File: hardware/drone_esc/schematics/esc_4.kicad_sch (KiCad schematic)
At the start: 32 parts, among them Q19 BSC016N04LS, Q20 BSC016N04LS, Q21 BSC016N04LS, Q22 BSC016N04LS, Q23 BSC016N04LS, Q24 BSC016N04LS, U10 FD6288Q

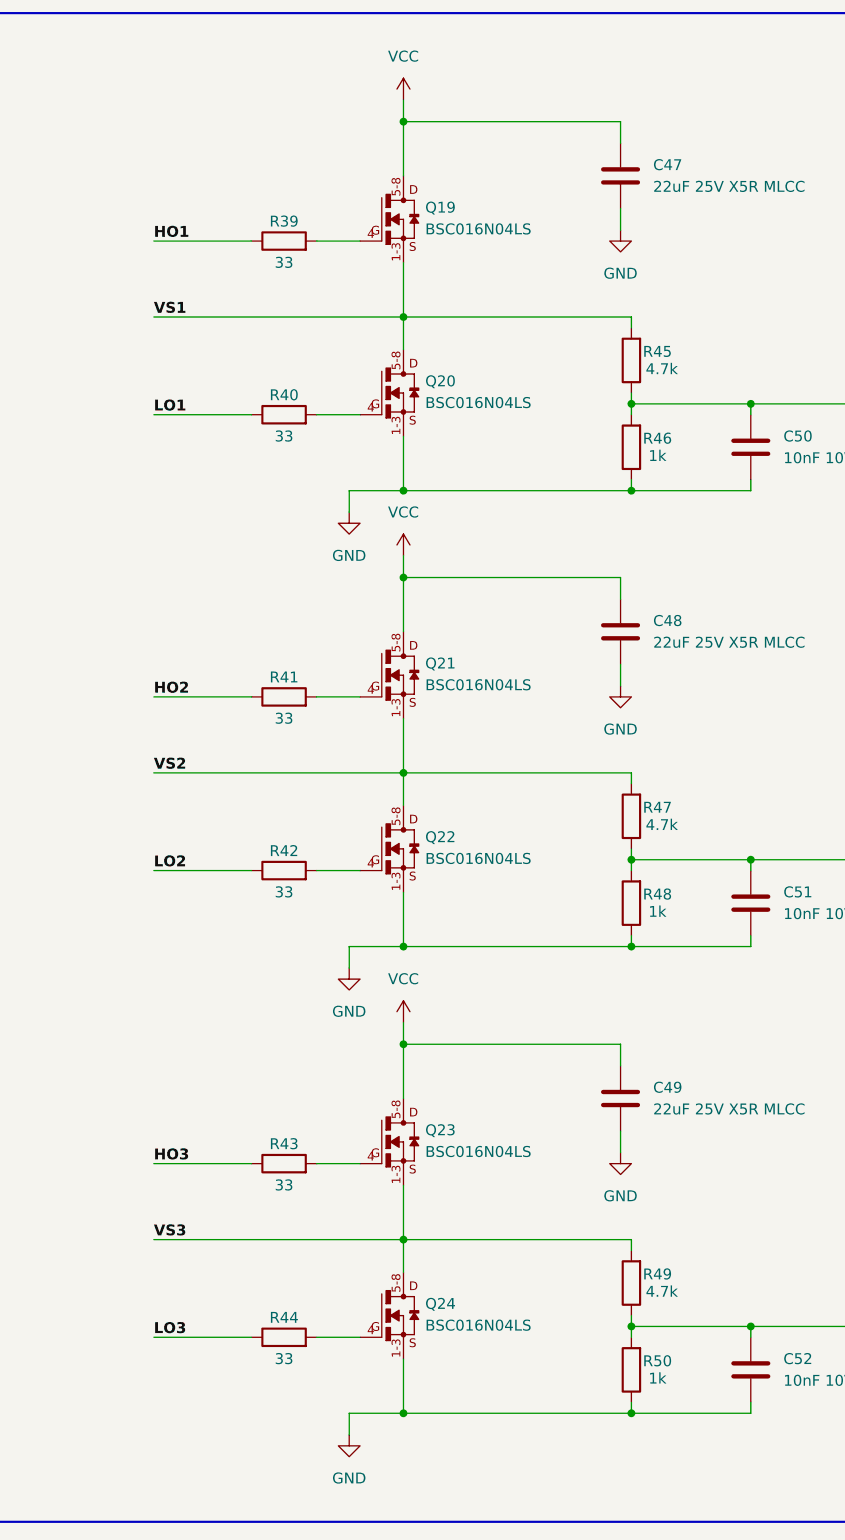
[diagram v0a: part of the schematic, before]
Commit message: replaced some of the schematics
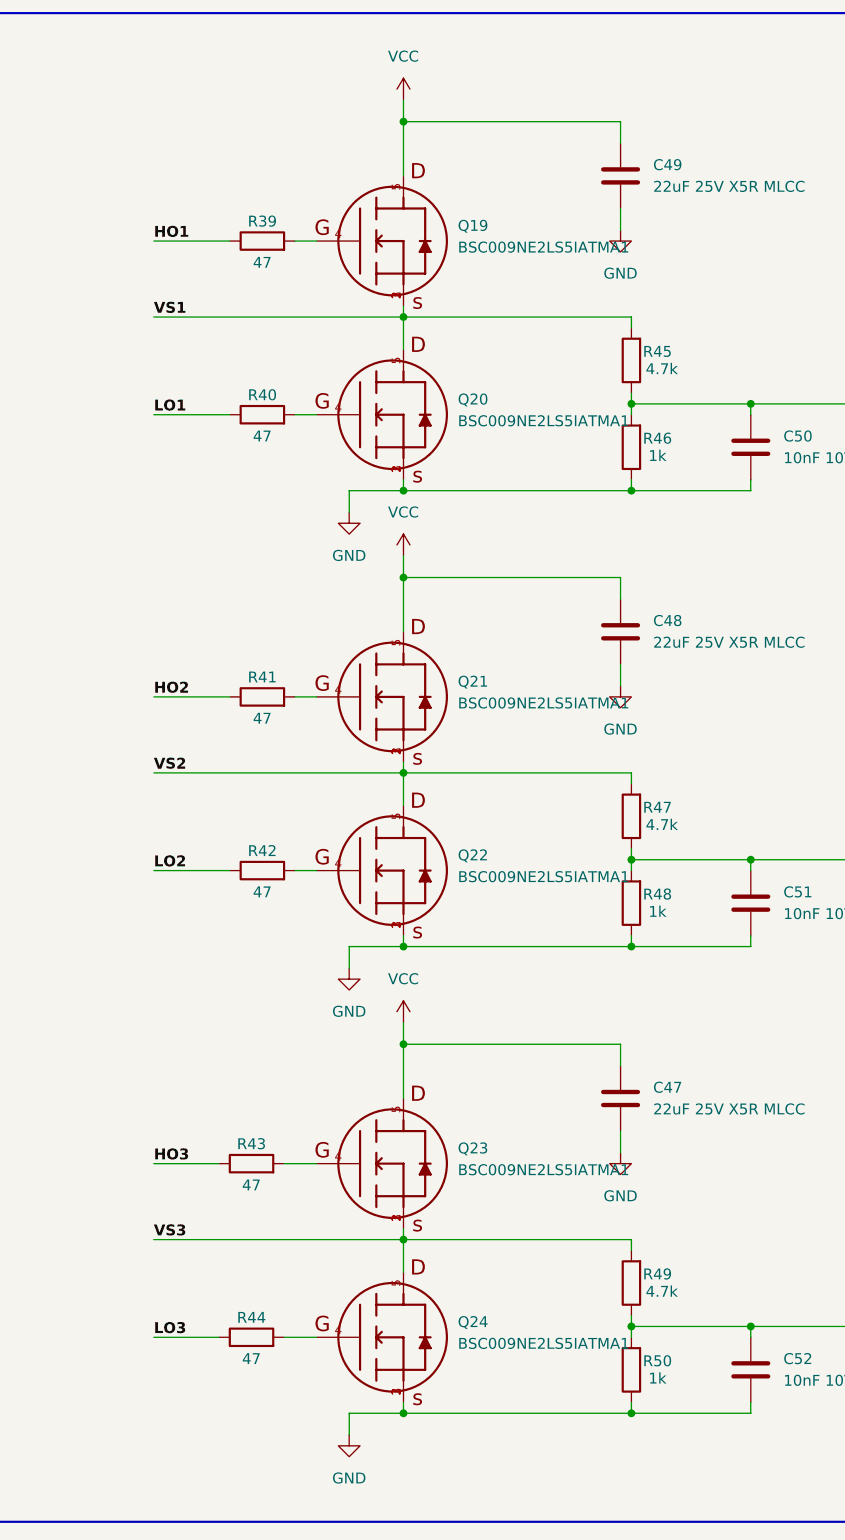
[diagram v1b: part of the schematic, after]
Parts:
- removed Q19, Q20, Q21, Q22, Q23, Q24: BSC016N04LS, Drone_components:BSC016N04LS, symbol Drone_components:BSC016N04LS
- added Q19, Q20, Q21, Q22, Q23, Q24: BSC009NE2LS5IATMA1, Drone_components:BSC093N04LSGATMA1, symbol Drone_components:BSC009NE2LS5IATMA1
- C47, C48, C49: footprint Capacitor_SMD:C_1210_3225Metric -> Capacitor_SMD:C_0805_2012Metric; JLCPCB part C12891 -> C45783
- R39, R40, R41, R42, R43, R44: value 33 -> 47
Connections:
- net GND: now also Q20.1, Q20.2, Q20.3, Q22.1, Q22.2, Q22.3, Q24.1, Q24.2, Q24.3
- net VCC: now also Q19.5, Q21.5, Q23.5
- net VS1: now also Q19.1, Q19.2, Q19.3, Q20.5
- net VS2: now also Q21.1, Q21.2, Q21.3, Q22.5
- net VS3: now also Q23.1, Q23.2, Q23.3, Q24.5
- net at R43.2: now also Q23.4
- net at R40.2: now also Q20.4
- net at R39.2: now also Q19.4
- net at R41.2: now also Q21.4
- net at R44.2: now also Q24.4
- net at R42.2: now also Q22.4
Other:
- moved on the sheet: R39, R40, R41, R42, R43, R44
